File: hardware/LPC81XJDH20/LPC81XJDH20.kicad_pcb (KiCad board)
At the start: 2 copper layers, 18.7 x 26.2 mm, 20 parts, among them J1 LPC81XJDH20_breakout_left, J2 JTAG_2X05, J3 LPC81XJDH20_breakout_right, U3 LPC812M101JDH20, Y1 12MHz

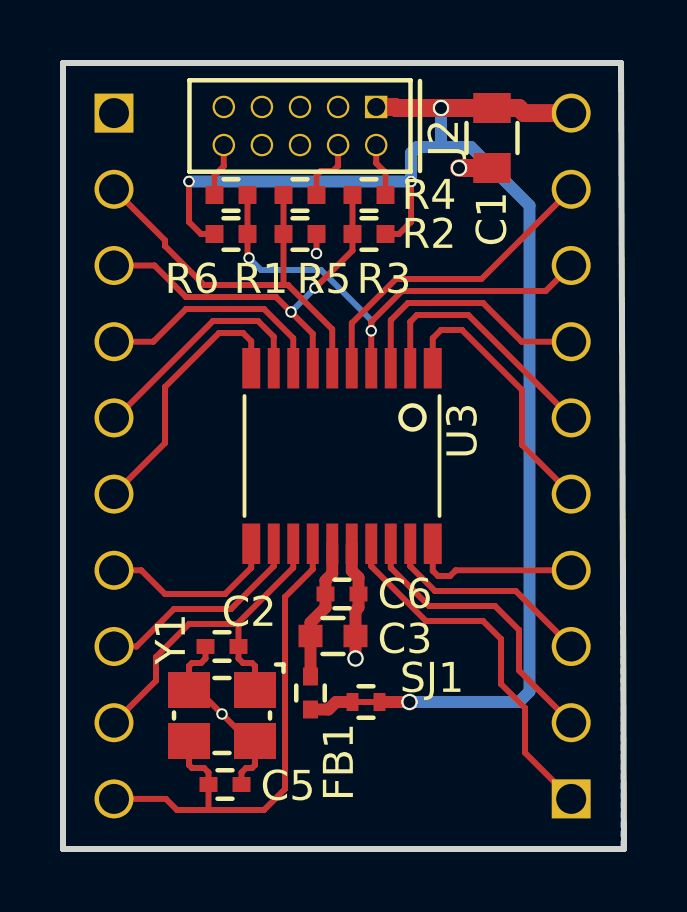
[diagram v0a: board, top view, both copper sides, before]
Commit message: various beauty changes
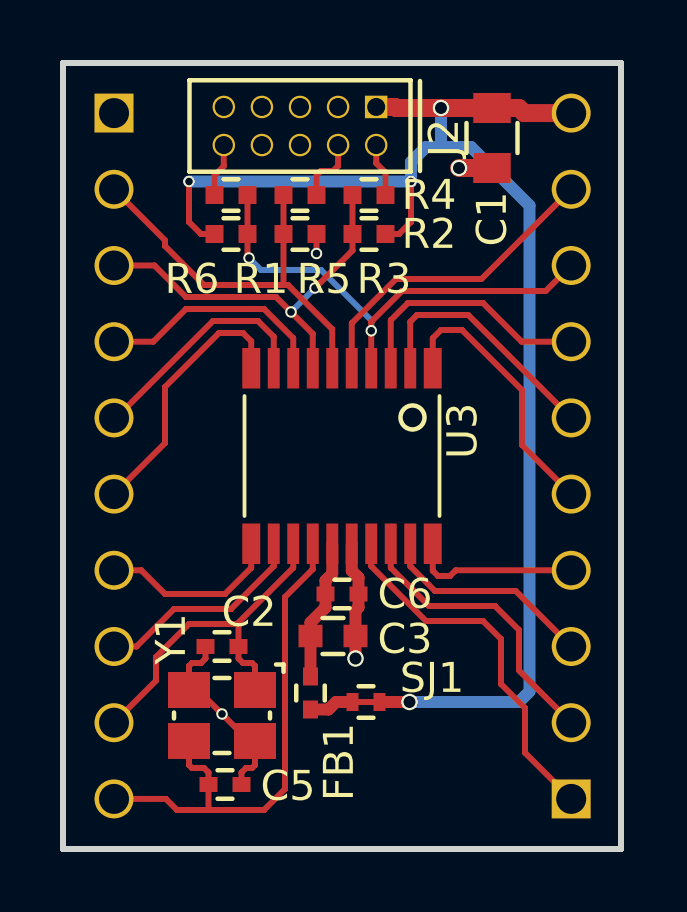
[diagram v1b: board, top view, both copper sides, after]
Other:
- board size 18.7 x 26.2 mm -> 18.6 x 26.2 mm
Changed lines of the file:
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@@
     (46 B.CrtYd user)
     (47 F.CrtYd user)
-    (48 B.Fab user hide)
-    (49 F.Fab user hide)
+    (48 B.Fab user)
+    (49 F.Fab user)
   )
   (setup
-    (last_trace_width 0.4)
+    (last_trace_width 0.1524)
     (user_trace_width 0.1524)
     (user_trace_width 0.2)
@@
       (effects (font (size 1 1) (thickness 0.15)) (justify left bottom))
     )
-    (fp_text value LPC812M101JDH20 (at 4.6 3.1 270) (layer F.Fab)
+    (fp_text value LPC812M101JDH20 (at 4.6 3.1 270) (layer F.Fab) hide
       (effects (font (size 1 1) (thickness 0.15)) (justify left bottom))
     )
@@
       (effects (font (size 1 1) (thickness 0.15)) (justify mirror))
     )
-    (fp_text value LPC81XJDH20_breakout_left (at 0 -2.1 270) (layer B.Fab)
+    (fp_text value LPC81XJDH20_breakout_left (at 0 -2.1 270) (layer B.Fab) hide
       (effects (font (size 1 1) (thickness 0.15)) (justify mirror))
     )
@@
       (effects (font (size 1 1) (thickness 0.15)) (justify mirror))
     )
-    (fp_text value LPC81XJDH20_breakout_right (at 0 -2.1 270) (layer B.Fab)
+    (fp_text value LPC81XJDH20_breakout_right (at 0 -2.1 270) (layer B.Fab) hide
       (effects (font (size 1 1) (thickness 0.15)) (justify mirror))
     )
@@
   )
   (gr_line (start 125.3 114.7) (end 125.3 88.5) (layer Edge.Cuts) (width 0.2))
-  (gr_line (start 144 114.7) (end 125.3 114.7) (layer Edge.Cuts) (width 0.2))
-  (gr_line (start 143.9 88.5) (end 144 114.7) (layer Edge.Cuts) (width 0.2))
+  (gr_line (start 143.9 114.7) (end 125.3 114.7) (layer Edge.Cuts) (width 0.2))
+  (gr_line (start 143.9 88.5) (end 143.9 114.7) (layer Edge.Cuts) (width 0.2))
   (gr_line (start 125.3 88.5) (end 143.9 88.5) (layer Edge.Cuts) (width 0.2))
   (segment (start 139.6 92) (end 138.5 92) (width 0.6) (layer F.Cu) (net 1))
@@
   (segment (start 136.9 93.8) (end 136.9 92.45) (width 0.2) (layer F.Cu) (net 2))
   (segment (start 129.5 92.45) (end 136.9 92.45) (width 0.4) (layer B.Cu) (net 2))
-  (segment (start 136.9 92.45) (end 136.9 91.5) (width 0.4) (layer B.Cu) (net 2))
-  (segment (start 136.9 91.5) (end 137.1 91.3) (width 0.4) (layer B.Cu) (net 2))
-  (segment (start 137.1 91.3) (end 137.9 91.3) (width 0.4) (layer B.Cu) (net 2))
   (segment (start 137.9 90.3) (end 137.9 91.3) (width 0.4) (layer B.Cu) (net 2))
   (segment (start 139.6 90) (end 140.5 90) (width 0.6) (layer F.Cu) (net 2))
@@
   (segment (start 136.85 109.8) (end 140.5 109.8) (width 0.4) (layer B.Cu) (net 2))
   (segment (start 140.5 109.8) (end 140.85 109.45) (width 0.4) (layer B.Cu) (net 2))
+  (segment (start 137.4 91.3) (end 137.9 91.3) (width 0.4) (layer B.Cu) (net 2))
+  (segment (start 136.9 92.45) (end 136.9 91.8) (width 0.4) (layer B.Cu) (net 2))
+  (segment (start 136.9 91.8) (end 137.4 91.3) (width 0.4) (layer B.Cu) (net 2))
   (segment (start 128.4 108.3) (end 128.4 109.09) (width 0.2) (layer F.Cu) (net 3))
   (segment (start 129.5 107.2) (end 128.4 108.3) (width 0.2) (layer F.Cu) (net 3))
@@
   (zone (net 1) (net_name VSS) (layer B.Cu) (hatch edge 0.508)
     (connect_pads (clearance 0.3))
-    (min_thickness 0.2)
-    (fill yes (arc_segments 16) (thermal_gap 0.3) (thermal_bridge_width 0.3))
+    (min_thickness 0.3)
+    (fill yes (arc_segments 16) (thermal_gap 0.3) (thermal_bridge_width 0.4))
     (polygon
       (pts
@@
   (zone (net 1) (net_name VSS) (layer F.Cu) (hatch edge 0.508)
     (connect_pads (clearance 0.3))
-    (min_thickness 0.254)
-    (fill yes (arc_segments 16) (thermal_gap 0.3) (thermal_bridge_width 0.3))
+    (min_thickness 0.3)
+    (fill yes (arc_segments 16) (thermal_gap 0.3) (thermal_bridge_width 0.4))
     (polygon
       (pts
-        (xy 125.3 88.5) (xy 143.9 88.5) (xy 144 114.7) (xy 125.3 114.7)
+        (xy 125.3 88.5) (xy 143.9 88.5) (xy 143.9 114.7) (xy 125.3 114.7)
       )
     )
